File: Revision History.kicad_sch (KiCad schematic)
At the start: 0 parts

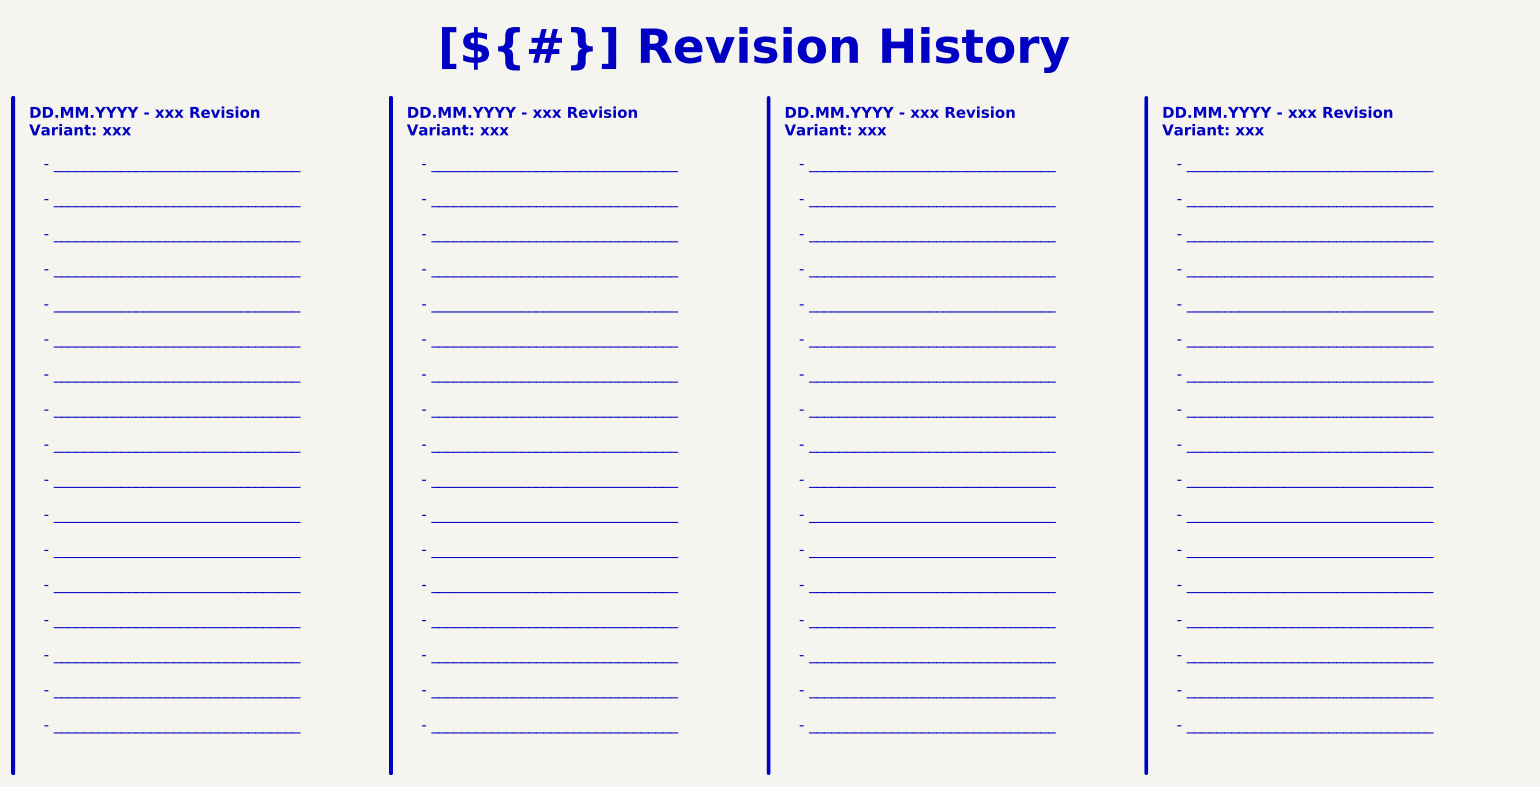
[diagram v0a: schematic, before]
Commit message: Finished 65% of schematics
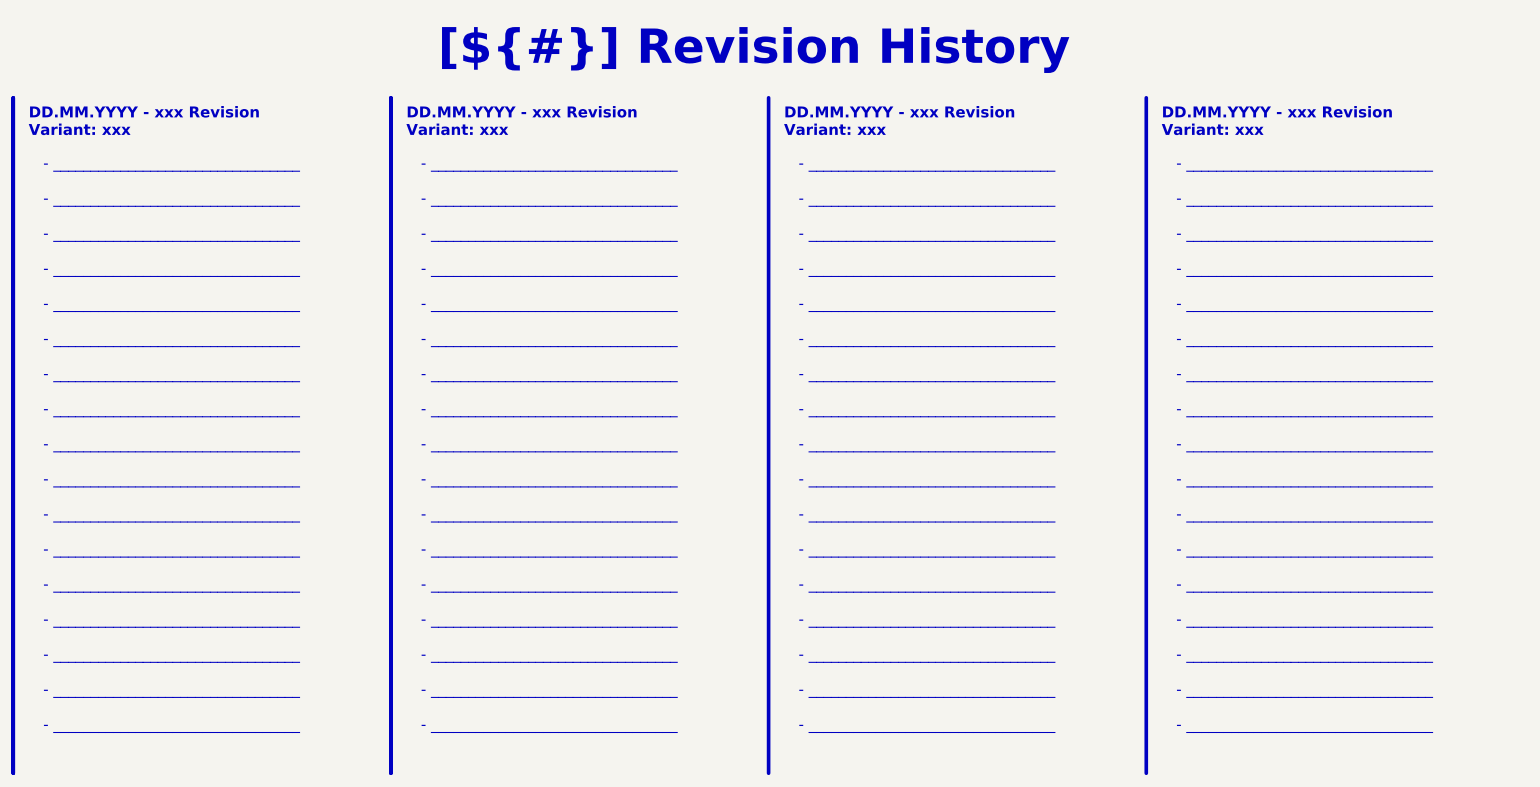
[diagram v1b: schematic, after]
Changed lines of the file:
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@@
 (kicad_sch
-	(version 20231120)
+	(version 20250114)
 	(generator "eeschema")
-	(generator_version "8.0")
+	(generator_version "9.0")
 	(paper "A4")
 	(title_block
@@
 		(company "${COMPANY}")
 	)
-	(polyline
-		(pts
-			(xy 19.05 31.75) (xy 19.05 149.86)
-		)
-		(stroke
-			(width 0.635)
-			(type default)
-			(color 0 0 0 1)
-		)
-	)
-	(polyline
-		(pts
-			(xy 85.09 31.75) (xy 85.09 149.86)
-		)
-		(stroke
-			(width 0.635)
-			(type default)
-			(color 0 0 0 1)
-		)
-	)
-	(polyline
-		(pts
-			(xy 85.09 31.75) (xy 85.09 149.86)
-		)
-		(stroke
-			(width 0.635)
-			(type default)
-			(color 0 0 0 1)
-		)
-	)
-	(polyline
-		(pts
-			(xy 151.13 31.75) (xy 151.13 149.86)
-		)
-		(stroke
-			(width 0.635)
-			(type default)
-			(color 0 0 0 1)
-		)
-	)
-	(polyline
-		(pts
-			(xy 19.05 31.75) (xy 19.05 149.86)
-		)
-		(stroke
-			(width 0.635)
-			(type default)
-			(color 0 0 0 1)
-		)
-	)
-	(polyline
-		(pts
-			(xy 217.17 31.75) (xy 217.17 149.86)
-		)
-		(stroke
-			(width 0.635)
-			(type default)
-			(color 0 0 0 1)
-		)
-	)
 	(text_box "- _________________________________\n\n- _________________________________\n\n- _________________________________\n\n- _________________________________\n\n- _________________________________\n\n- _________________________________\n\n- _________________________________\n\n- _________________________________\n\n- _________________________________\n\n- _________________________________\n\n- _________________________________\n\n- _________________________________\n\n- _________________________________\n\n- _________________________________\n\n- _________________________________\n\n- _________________________________\n\n- _________________________________"
 		(exclude_from_sim no)
 		(at 220.98 40.64 0)
 		(size 58.42 115.57)
+		(margins 1.4287 1.4287 1.4287 1.4287)
 		(stroke
 			(width -0.0001)
@@
 		(at 86.36 31.75 0)
 		(size 57.15 7.62)
+		(margins 1.4287 1.4287 1.4287 1.4287)
 		(stroke
 			(width -0.0001)
@@
 		(at 80.01 16.51 0)
 		(size 137.16 12.7)
+		(margins 4.4999 4.4999 4.4999 4.4999)
 		(stroke
 			(width -0.0001)
@@
 		(at 152.4 31.75 0)
 		(size 57.15 7.62)
+		(margins 1.4287 1.4287 1.4287 1.4287)
 		(stroke
 			(width -0.0001)
@@
 		(at 22.86 40.64 0)
 		(size 58.42 115.57)
+		(margins 1.4287 1.4287 1.4287 1.4287)
 		(stroke
 			(width -0.0001)
@@
 		(at 154.94 40.64 0)
 		(size 58.42 115.57)
+		(margins 1.4287 1.4287 1.4287 1.4287)
 		(stroke
 			(width -0.0001)
@@
 		(at 20.32 31.75 0)
 		(size 57.15 7.62)
+		(margins 1.4287 1.4287 1.4287 1.4287)
 		(stroke
 			(width -0.0001)
@@
 		(at 88.9 40.64 0)
 		(size 58.42 115.57)
+		(margins 1.4287 1.4287 1.4287 1.4287)
 		(stroke
 			(width -0.0001)
@@
 		(at 218.44 31.75 0)
 		(size 57.15 7.62)
-		(stroke
-			(width -0.0001)
-			(type default)
-		)
-		(fill
-			(type none)
-		)
-		(effects
-			(font
-				(face "Arial")
-				(size 1.905 1.905)
-				(thickness 0.254)
-				(bold yes)
-			)
-			(justify left top)
-		)
-	)
+		(margins 1.4287 1.4287 1.4287 1.4287)
+		(stroke
+			(width -0.0001)
+			(type default)
+		)
+		(fill
+			(type none)
+		)
+		(effects
+			(font
+				(face "Arial")
+				(size 1.905 1.905)
+				(thickness 0.254)
+				(bold yes)
+			)
+			(justify left top)
+		)
+	)
+	(polyline
+		(pts
+			(xy 19.05 31.75) (xy 19.05 149.86)
+		)
+		(stroke
+			(width 0.635)
+			(type default)
+			(color 0 0 0 1)
+		)
+	)
+	(polyline
+		(pts
+			(xy 85.09 31.75) (xy 85.09 149.86)
+		)
+		(stroke
+			(width 0.635)
+			(type default)
+			(color 0 0 0 1)
+		)
+	)
+	(polyline
+		(pts
+			(xy 85.09 31.75) (xy 85.09 149.86)
+		)
+		(stroke
+			(width 0.635)
+			(type default)
+			(color 0 0 0 1)
+		)
+	)
+	(polyline
+		(pts
+			(xy 151.13 31.75) (xy 151.13 149.86)
+		)
+		(stroke
+			(width 0.635)
+			(type default)
+			(color 0 0 0 1)
+		)
+	)
+	(polyline
+		(pts
+			(xy 19.05 31.75) (xy 19.05 149.86)
+		)
+		(stroke
+			(width 0.635)
+			(type default)
+			(color 0 0 0 1)
+		)
+	)
+	(polyline
+		(pts
+			(xy 217.17 31.75) (xy 217.17 149.86)
+		)
+		(stroke
+			(width 0.635)
+			(type default)
+			(color 0 0 0 1)
+		)
+	)
